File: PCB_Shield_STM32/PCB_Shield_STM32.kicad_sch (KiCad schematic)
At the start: 51 parts, among them CN10 Conn_02x19_Odd_Even, CN11 Conn_01x02, CN12 Conn_01x02, CN5 Conn_01x10, CN6 Conn_01x08, CN7 Conn_02x19_Odd_Even, CN8 Conn_01x06, CN9 Conn_01x08, J1 Barrel_Jack_Switch, SW1 SW_SPST, U2 LM2903P

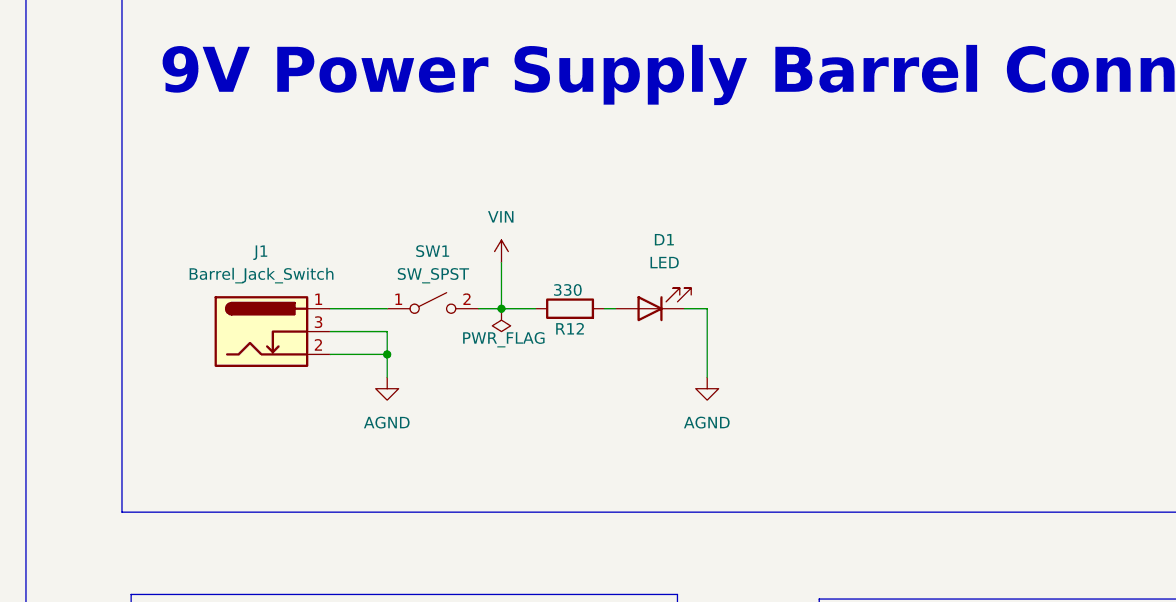
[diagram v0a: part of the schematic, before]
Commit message: PCB V1 Finalized
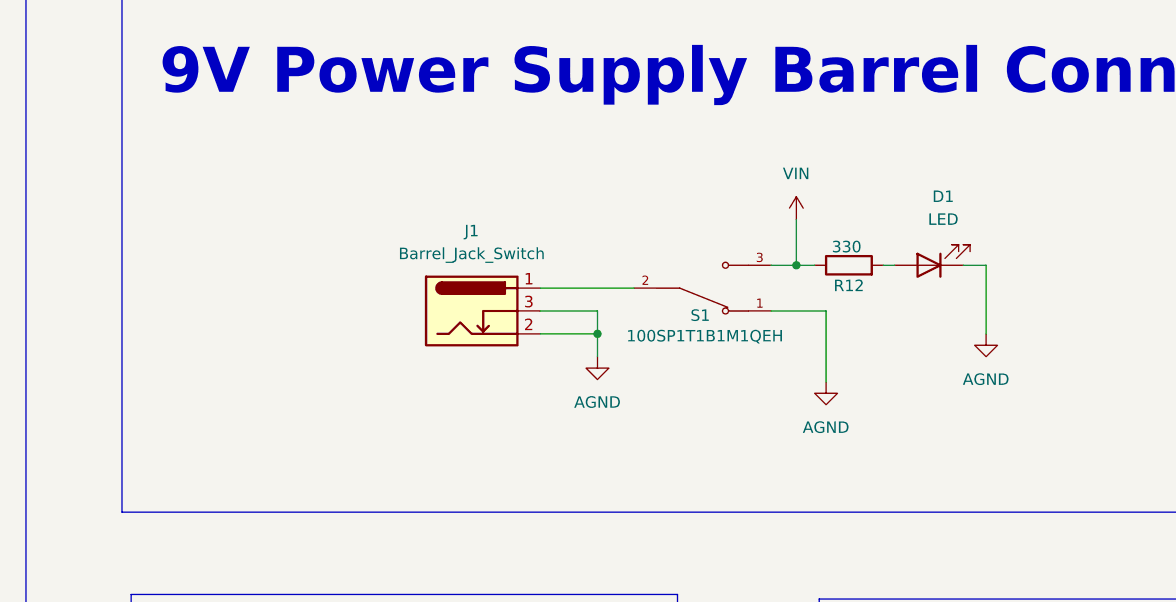
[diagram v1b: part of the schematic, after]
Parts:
- removed SW1: SW_SPST, Button_Switch_THT:SW_DIP_SPSTx01_Slide_9.78x4.72mm_W7.62mm_P2.54mm, symbol Switch:SW_SPST
- added S1: 100SP1T1B1M1QEH, 100SP1T1B1M1QEH:SW_100SP1T1B1M1QEH, symbol 100SP1T1B1M1QEH:100SP1T1B1M1QEH
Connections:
- net AGND: now also S1.1
- net VIN: now also S1.3
- net at J1.1: now also S1.2
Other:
- moved on the sheet: J1
